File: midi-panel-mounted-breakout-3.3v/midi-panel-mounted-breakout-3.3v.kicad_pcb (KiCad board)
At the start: 2 copper layers, 53 x 16.5 mm, 16 parts, among them J1 SD-50BV, J2 SD-50BV, J3 Conn_01x04_Male, U1 H11L1

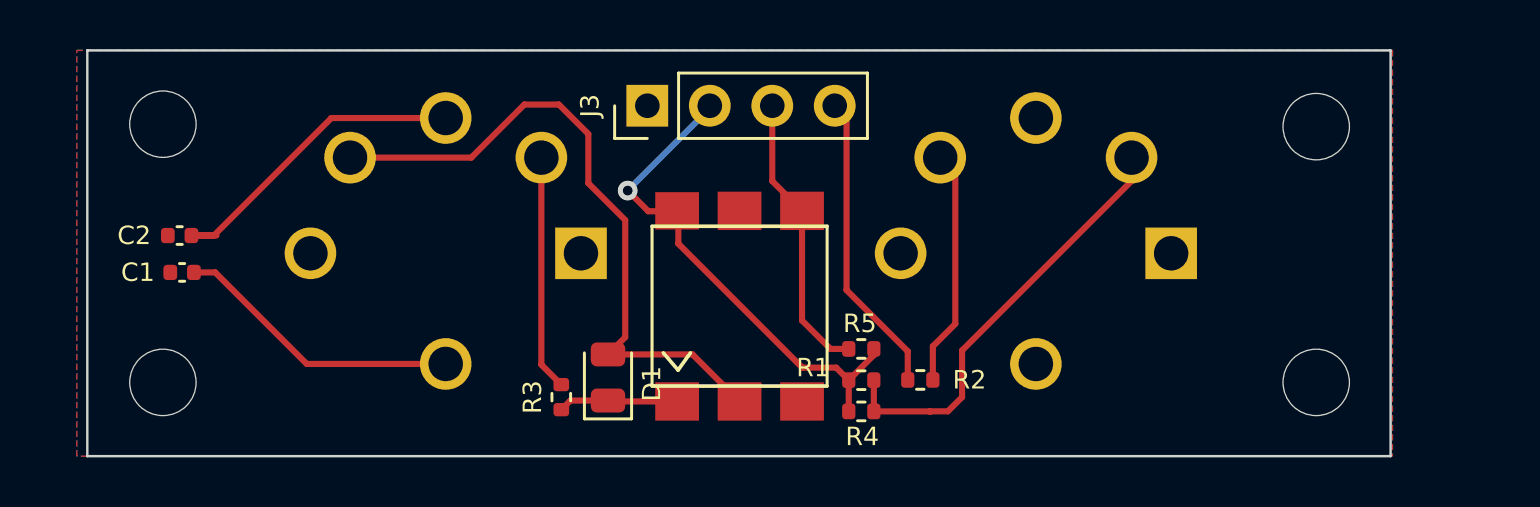
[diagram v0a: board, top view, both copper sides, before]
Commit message: WIP-changes
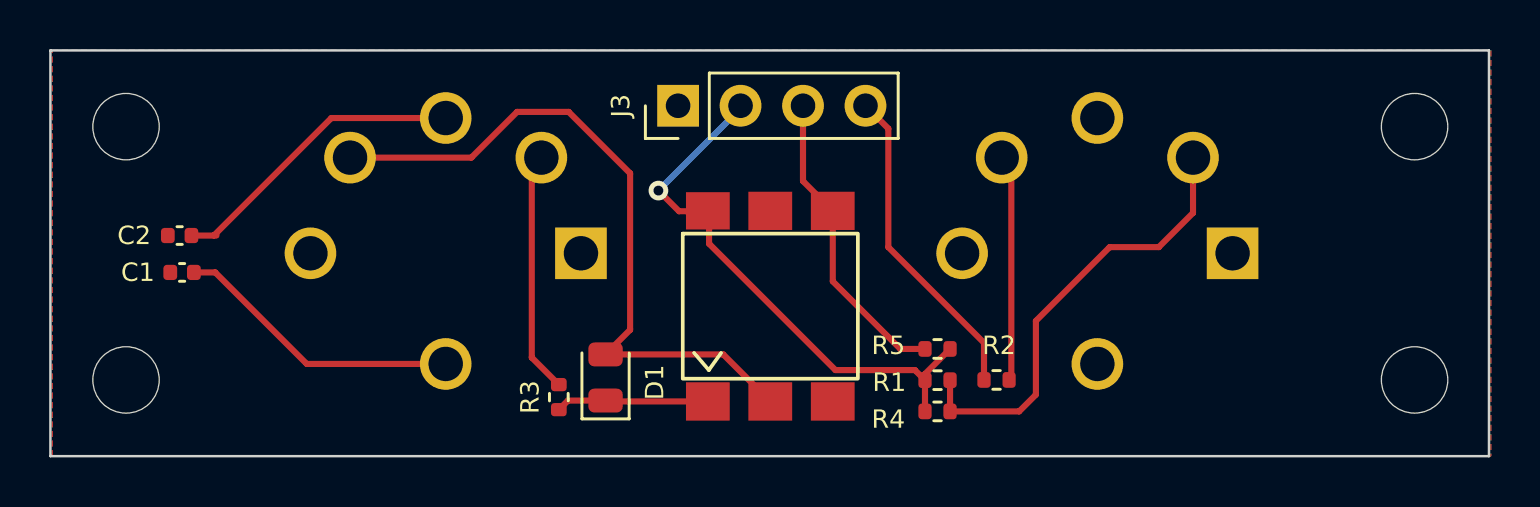
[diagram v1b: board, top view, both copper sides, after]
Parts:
- moved REF** 4.00 mm to (159.9, 73.4)
- moved REF** 4.00 mm to (159.9, 63.1)
- moved R1 3.10 mm to (140.5, 73.4)
- moved R2 3.10 mm to (142.9, 73.4), turned to 180 degrees
- moved R4 3.10 mm to (140.5, 74.7)
- moved R5 3.10 mm to (140.5, 72.1)
- moved J2 2.50 mm to (147.0, 68.2)
- moved REF** 1.50 mm to (107.5, 63.1)
- moved REF** 1.50 mm to (107.5, 73.4)
- moved J3 1.25 mm to (129.9, 62.2)
- moved U1 1.25 mm to (133.7, 70.4)
- moved R3 0.10 mm to (125.1, 74.1)
- moved D1 0.10 mm to (127.0, 73.3)
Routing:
- net +3V3: track 21.0 -> 22.4 mm
- net /Tx: track 12.6 -> 13.8 mm
- net /Rx: track 11.9 -> 12.8 mm
- net Net-(C2-Pad1): track 13.4 -> 12.5 mm
- net Net-(D1-Pad2): track 27.1 -> 28.0 mm
- net Net-(J2-Pad4): track 17.7 -> 18.5 mm
- net Net-(D1-Pad1): track 4.88 -> 5.68 mm
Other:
- board size 53 x 16.5 mm -> 58.5 x 16.5 mm
